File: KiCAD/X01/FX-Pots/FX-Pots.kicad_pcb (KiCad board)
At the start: 2 copper layers, 56 x 108 mm, 17 parts, among them J1 Conn_01x04, J2 Conn_01x03, U1 CD74HC4067M

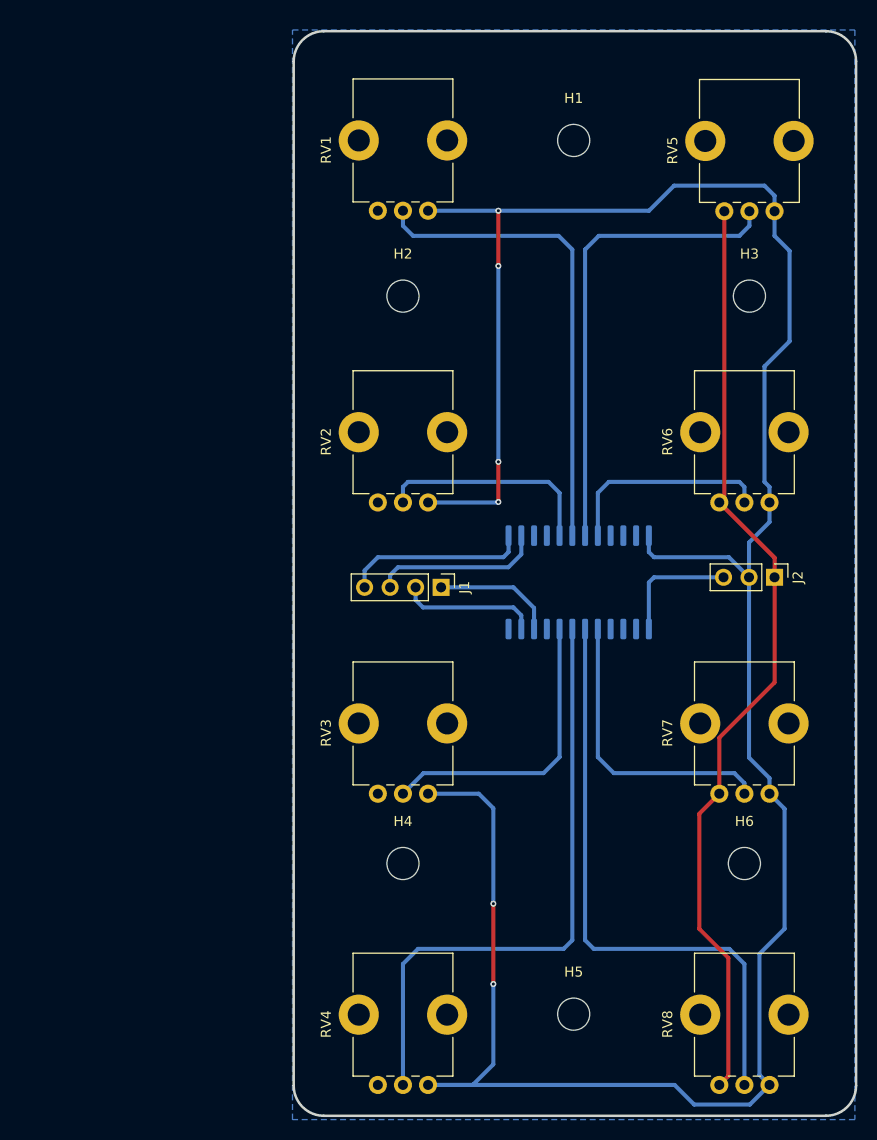
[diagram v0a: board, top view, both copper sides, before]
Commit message: fx pots
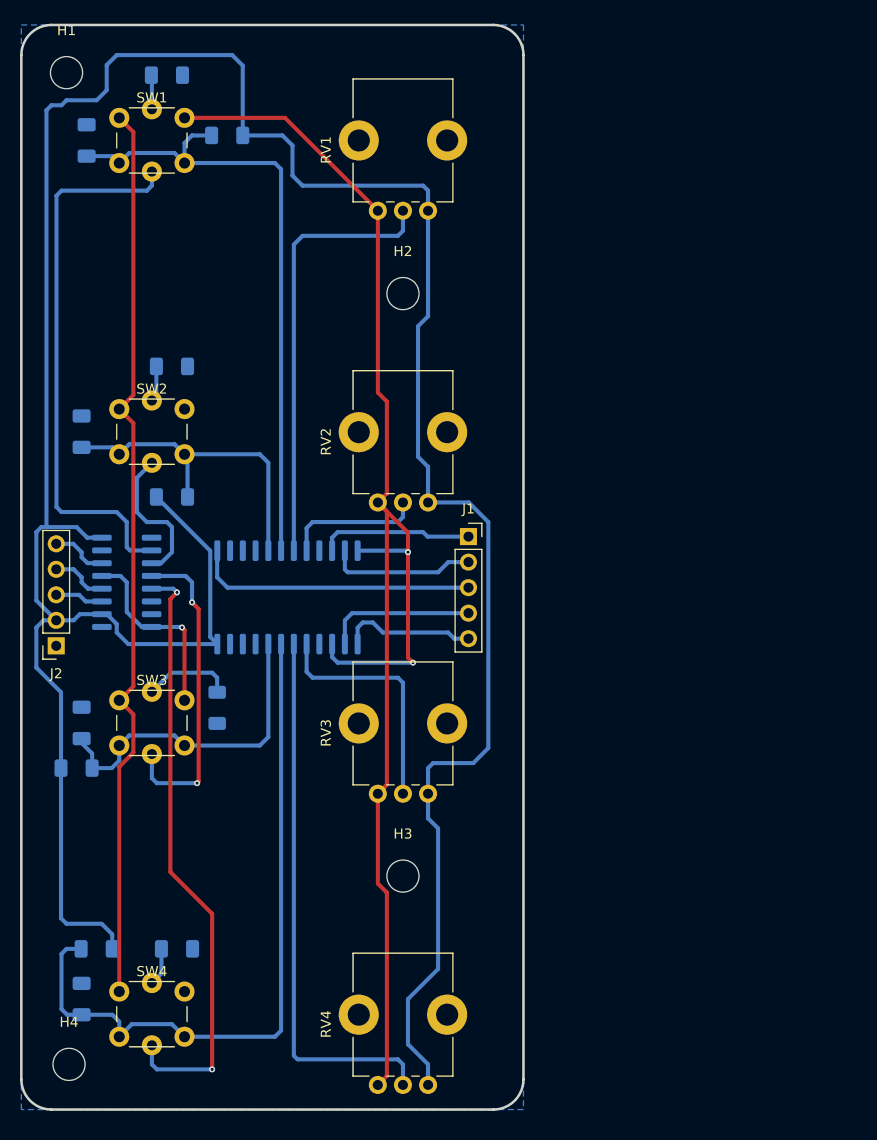
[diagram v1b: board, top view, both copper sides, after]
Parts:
- removed H5, H6: MountingHole_M3, MountingHole:MountingHole_3.2mm_M3
- removed RV5, RV6, RV7, RV8: R_Pot, Potentiometer_THT:Potentiometer_Bourns_PTV09A-1_Single_Vertical
- added C1: 1uF, Capacitor_SMD:C_1206_3216Metric_Pad1.33x1.80mm_HandSolder, B.Cu at (74.5, 51.0)
- added C2: 1uF, Capacitor_SMD:C_1206_3216Metric_Pad1.33x1.80mm_HandSolder, B.Cu at (74.0, 80.0)
- added C3: 1uF, Capacitor_SMD:C_1206_3216Metric_Pad1.33x1.80mm_HandSolder, B.Cu at (74.0, 109.0)
- added C4: 1uF, Capacitor_SMD:C_1206_3216Metric_Pad1.33x1.80mm_HandSolder, B.Cu at (74.0, 136.5)
- added R1: 220, PCM_Resistor_SMD_AKL:R_1206_3216Metric_Pad1.30x1.75mm_HandSolder, B.Cu at (82.5, 44.5)
- added R2: 220, PCM_Resistor_SMD_AKL:R_1206_3216Metric_Pad1.30x1.75mm_HandSolder, B.Cu at (83.0, 73.5)
- added R3: 220, PCM_Resistor_SMD_AKL:R_1206_3216Metric_Pad1.30x1.75mm_HandSolder, B.Cu at (87.5, 107.5)
- added R4: 220, PCM_Resistor_SMD_AKL:R_1206_3216Metric_Pad1.30x1.75mm_HandSolder, B.Cu at (83.5, 131.5)
- added R5: 10K, PCM_Resistor_SMD_AKL:R_1206_3216Metric_Pad1.30x1.75mm_HandSolder, B.Cu at (88.5, 50.5)
- added R6: 10K, PCM_Resistor_SMD_AKL:R_1206_3216Metric_Pad1.30x1.75mm_HandSolder, B.Cu at (83.0, 86.5)
- added R7: 10K, PCM_Resistor_SMD_AKL:R_1206_3216Metric_Pad1.30x1.75mm_HandSolder, B.Cu at (73.5, 113.5)
- added R8: 10K, PCM_Resistor_SMD_AKL:R_1206_3216Metric_Pad1.30x1.75mm_HandSolder, B.Cu at (75.5, 131.5)
- added SW1: SW_Push_LED, led-switch:SW_PUSH_6mm_LED, F.Cu at (81.0, 51.0)
- added SW2: SW_Push_LED, led-switch:SW_PUSH_6mm_LED, F.Cu at (81.0, 80.0)
- added SW3: SW_Push_LED, led-switch:SW_PUSH_6mm_LED, F.Cu at (81.0, 109.0)
- added SW4: SW_Push_LED, led-switch:SW_PUSH_6mm_LED, F.Cu at (81.0, 138.0)
- added U2: CD74HC4067M, Package_SO:SOIC-24W_7.5x15.4mm_P1.27mm, B.Cu at (94.5, 96.5)
- J1: value Conn_01x04 -> Conn_01x05; footprint Connector_PinHeader_2.54mm:PinHeader_1x04_P2.54mm_Vertical -> Connector_PinSocket_2.54mm:PinSocket_1x05_P2.54mm_Vertical
- J2: value Conn_01x03 -> Conn_01x05; footprint Connector_PinHeader_2.54mm:PinHeader_1x03_P2.54mm_Vertical -> Connector_PinSocket_2.54mm:PinSocket_1x05_P2.54mm_Vertical
- U1: value CD74HC4067M -> 74HC595; footprint Package_SO:SOIC-24W_7.5x15.4mm_P1.27mm -> Package_SO:SOIC-16_3.9x9.9mm_P1.27mm
- moved J2 71.8 mm to (71.5, 101.3), turned to 180 degrees
- moved H3 67.3 mm to (106.0, 124.2)
- moved H1 50.9 mm to (72.5, 44.2)
- moved U1 45.0 mm to (78.5, 95.0), turned to 180 degrees
- moved H4 38.8 mm to (72.8, 143.0)
- moved J1 5.74 mm to (112.5, 90.5), turned to 0 degrees
- moved H2 0.25 mm to (106.0, 66.2)
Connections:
- J1 pad 3: MPLEX-S2 -> MPLEX-AP
- J1 pad 4: MPLEX-S3 -> MPLEX-S2
- J2 pad 3: MPLEX-AP -> SRCLK
- U1 pad 1: MPLEX-AP -> unconnected-(U1-QB-Pad1)
- U1 pad 10: MPLEX-S0 -> +5V
- U1 pad 11: MPLEX-S1 -> SRCLK
- U1 pad 12: GND -> FX-LED-LATCH
- U1 pad 13: MPLEX-S3 -> GND
- U1 pad 14: MPLEX-S2 -> FX-LED-SIG
- U1 pad 15: GND -> unconnected-(U1-QA-Pad15)
- U1 pad 16: unconnected-(U1-I15-Pad16) -> +5V
- U1 pad 2: unconnected-(U1-I7-Pad2) -> FX-LED-1
- U1 pad 3: unconnected-(U1-I6-Pad3) -> FX-LED-2
- U1 pad 4: unconnected-(U1-I5-Pad4) -> FX-LED-3
- U1 pad 5: POT7 -> FX-LED-4
- U1 pad 6: POT8 -> unconnected-(U1-QG-Pad6)
- U1 pad 7: POT4 -> unconnected-(U1-QH-Pad7)
- U1 pad 8: POT3 -> GND
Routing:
- net GND: track 94.2 -> 254.1 mm, vias 0 -> 3
- net FXSW4: track 0.00 -> 71.3 mm
- net FXSW1: track 0.00 -> 63.7 mm
- net FX-LED-4: track 0.00 -> 60.3 mm, vias 0 -> 2
- net POT8: track 59.9 -> 0.00 mm
- net FX-LED-1: track 0.00 -> 55.0 mm
- net POT5: track 47.3 -> 0.00 mm
- net +5V: track 254.4 -> 288.1 mm, vias 6 -> 0
- net FXSW2: track 0.00 -> 33.2 mm
- net FXSW3: track 0.00 -> 33.2 mm
- net FX-LED-3: track 0.00 -> 31.7 mm, vias 0 -> 2
- net POT7: track 29.5 -> 0.00 mm
- net POT6: track 21.1 -> 0.00 mm
- net MPLEX-AP: track 12.3 -> 28.1 mm
- net FX-LED-2: track 0.00 -> 14.6 mm
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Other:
- board size 56 x 108 mm -> 50 x 108 mm
